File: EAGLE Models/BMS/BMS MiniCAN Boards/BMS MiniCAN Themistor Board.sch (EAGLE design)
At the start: 112 parts, among them IC1 AT90CAN128, IC2 MCP2551SO8, IC3 NUP2105L, U1 0ZCH0050FF2G

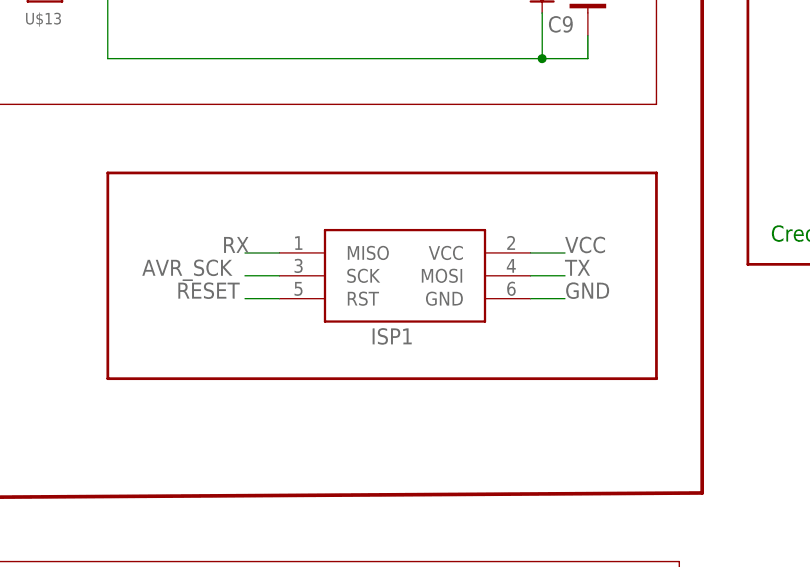
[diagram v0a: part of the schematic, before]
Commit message: Finished First Revision of Thermistor Board
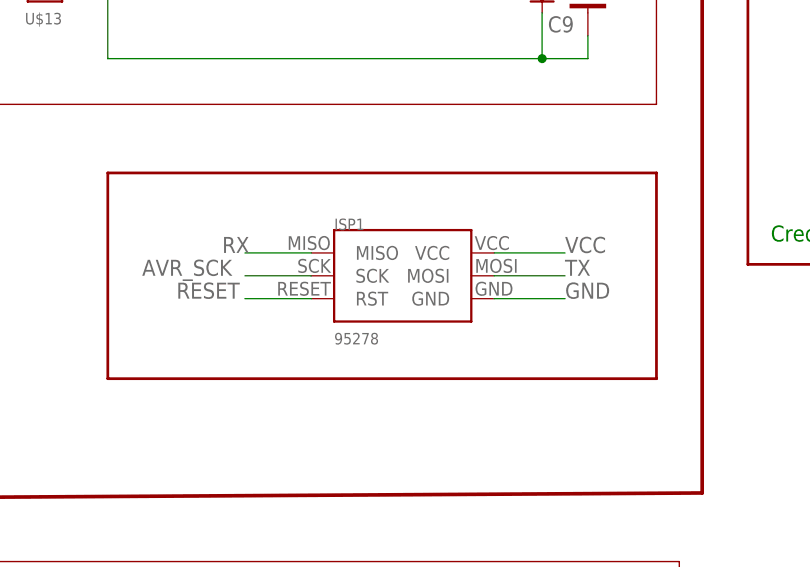
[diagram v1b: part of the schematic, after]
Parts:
- ISP1: value AVRISP-6 -> 95278; device adafruit:AVRISP-6 -> con-amphenol:95278
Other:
- moved on the sheet: ISP1
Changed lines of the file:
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@@
 <setting verticaltext="up"/>
 </settings>
-<grid distance="1.27" unitdist="mm" unit="mm" style="lines" multiple="1" display="no" altdistance="0.3175" altunitdist="mm" altunit="mm"/>
+<grid distance="0.1" unitdist="inch" unit="inch" style="lines" multiple="1" display="no" altdistance="0.01" altunitdist="inch" altunit="inch"/>
 <layers>
 <layer number="1" name="Top" color="4" fill="1" visible="no" active="no"/>
@@
 <part name="D2" library="BMS Lbr" deviceset="DFLS1100" device=""/>
 <part name="U$13" library="BMS Lbr" deviceset="0039300040" device=""/>
-<part name="ISP1" library="adafruit" deviceset="AVRISP" device="-6"/>
 <part name="C10" library="rcl" deviceset="C-US" device="C0805" value="0.1uF"/>
 <part name="U$14" library="BMS Lbr" deviceset="AX-16.000MBGE-T" device=""/>
+<part name="ISP1" library="con-amphenol" deviceset="95278" device=""/>
 </parts>
 <sheets>
@@
 <instance part="D2" gate="G$1" x="195.58" y="180.34"/>
 <instance part="U$13" gate="G$1" x="81.28" y="55.88" rot="R180"/>
-<instance part="ISP1" gate="G$1" x="120.65" y="19.05"/>
 <instance part="C10" gate="G$1" x="294.64" y="160.02" rot="R90"/>
 <instance part="U$14" gate="G$1" x="306.07" y="171.45" rot="R90"/>
+<instance part="ISP1" gate="G$1" x="121.666" y="19.05"/>
 </instances>
 <busses>
@@
 </segment>
 <segment>
+<label x="139.7" y="21.59" size="1.778" layer="95"/>
 <pinref part="ISP1" gate="G$1" pin="VCC"/>
-<wire x1="135.89" y1="21.59" x2="139.7" y2="21.59" width="0.1524" layer="91"/>
-<label x="139.7" y="21.59" size="1.778" layer="95"/>
+<wire x1="131.826" y1="21.59" x2="139.7" y2="21.59" width="0.1524" layer="91"/>
 </segment>
 <segment>
@@
 </segment>
 <segment>
+<label x="139.7" y="16.51" size="1.778" layer="95"/>
 <pinref part="ISP1" gate="G$1" pin="GND"/>
-<wire x1="135.89" y1="16.51" x2="139.7" y2="16.51" width="0.1524" layer="91"/>
-<label x="139.7" y="16.51" size="1.778" layer="95"/>
+<wire x1="131.826" y1="16.51" x2="139.7" y2="16.51" width="0.1524" layer="91"/>
 </segment>
 </net>
@@
 </segment>
 <segment>
+<wire x1="111.506" y1="16.51" x2="104.14" y2="16.51" width="0.1524" layer="91"/>
+<label x="96.52" y="16.51" size="1.778" layer="95"/>
 <pinref part="ISP1" gate="G$1" pin="RST"/>
-<wire x1="107.95" y1="16.51" x2="104.14" y2="16.51" width="0.1524" layer="91"/>
-<label x="96.52" y="16.51" size="1.778" layer="95"/>
 </segment>
 </net>
@@
 </segment>
 <segment>
+<label x="139.7" y="19.05" size="1.778" layer="95"/>
 <pinref part="ISP1" gate="G$1" pin="MOSI"/>
-<wire x1="135.89" y1="19.05" x2="139.7" y2="19.05" width="0.1524" layer="91"/>
-<label x="139.7" y="19.05" size="1.778" layer="95"/>
+<wire x1="131.826" y1="19.05" x2="139.7" y2="19.05" width="0.1524" layer="91"/>
 </segment>
 </net>
@@
 </segment>
 <segment>
+<wire x1="111.506" y1="21.59" x2="104.14" y2="21.59" width="0.1524" layer="91"/>
+<label x="101.6" y="21.59" size="1.778" layer="95"/>
 <pinref part="ISP1" gate="G$1" pin="MISO"/>
-<wire x1="107.95" y1="21.59" x2="104.14" y2="21.59" width="0.1524" layer="91"/>
-<label x="101.6" y="21.59" size="1.778" layer="95"/>
 </segment>
 </net>
@@
 </segment>
 <segment>
+<wire x1="111.506" y1="19.05" x2="104.14" y2="19.05" width="0.1524" layer="91"/>
+<label x="92.71" y="19.05" size="1.778" layer="95"/>
 <pinref part="ISP1" gate="G$1" pin="SCK"/>
-<wire x1="107.95" y1="19.05" x2="104.14" y2="19.05" width="0.1524" layer="91"/>
-<label x="92.71" y="19.05" size="1.778" layer="95"/>
-</segment>
-</net>
+</segment>
+</net>
